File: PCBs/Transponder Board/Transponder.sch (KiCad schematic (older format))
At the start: 17 parts

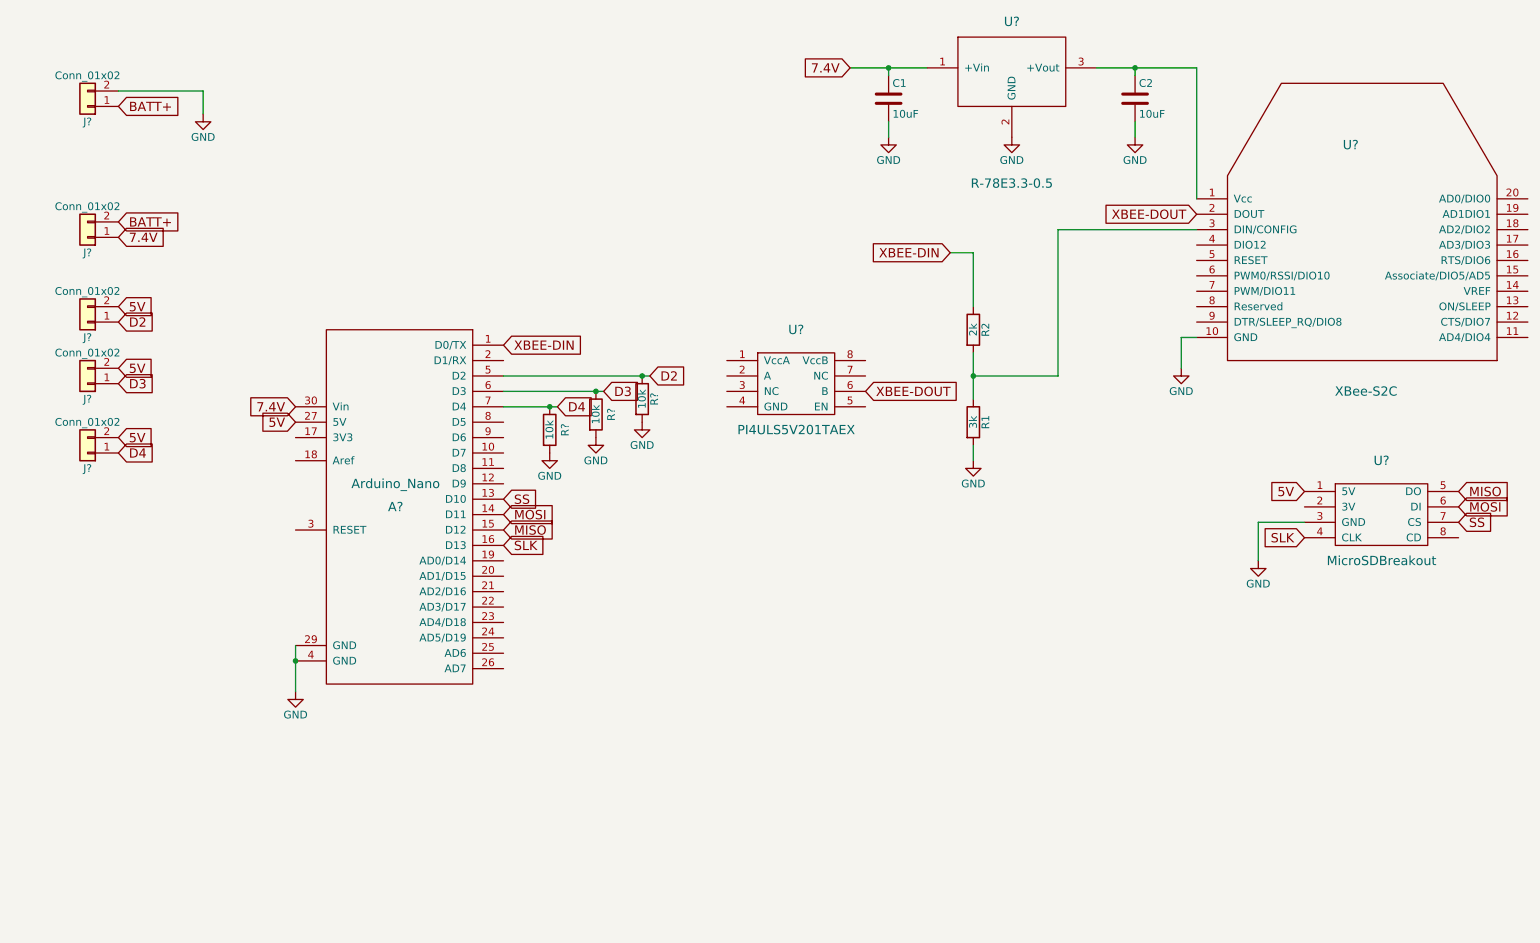
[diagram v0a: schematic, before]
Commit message: transponder board
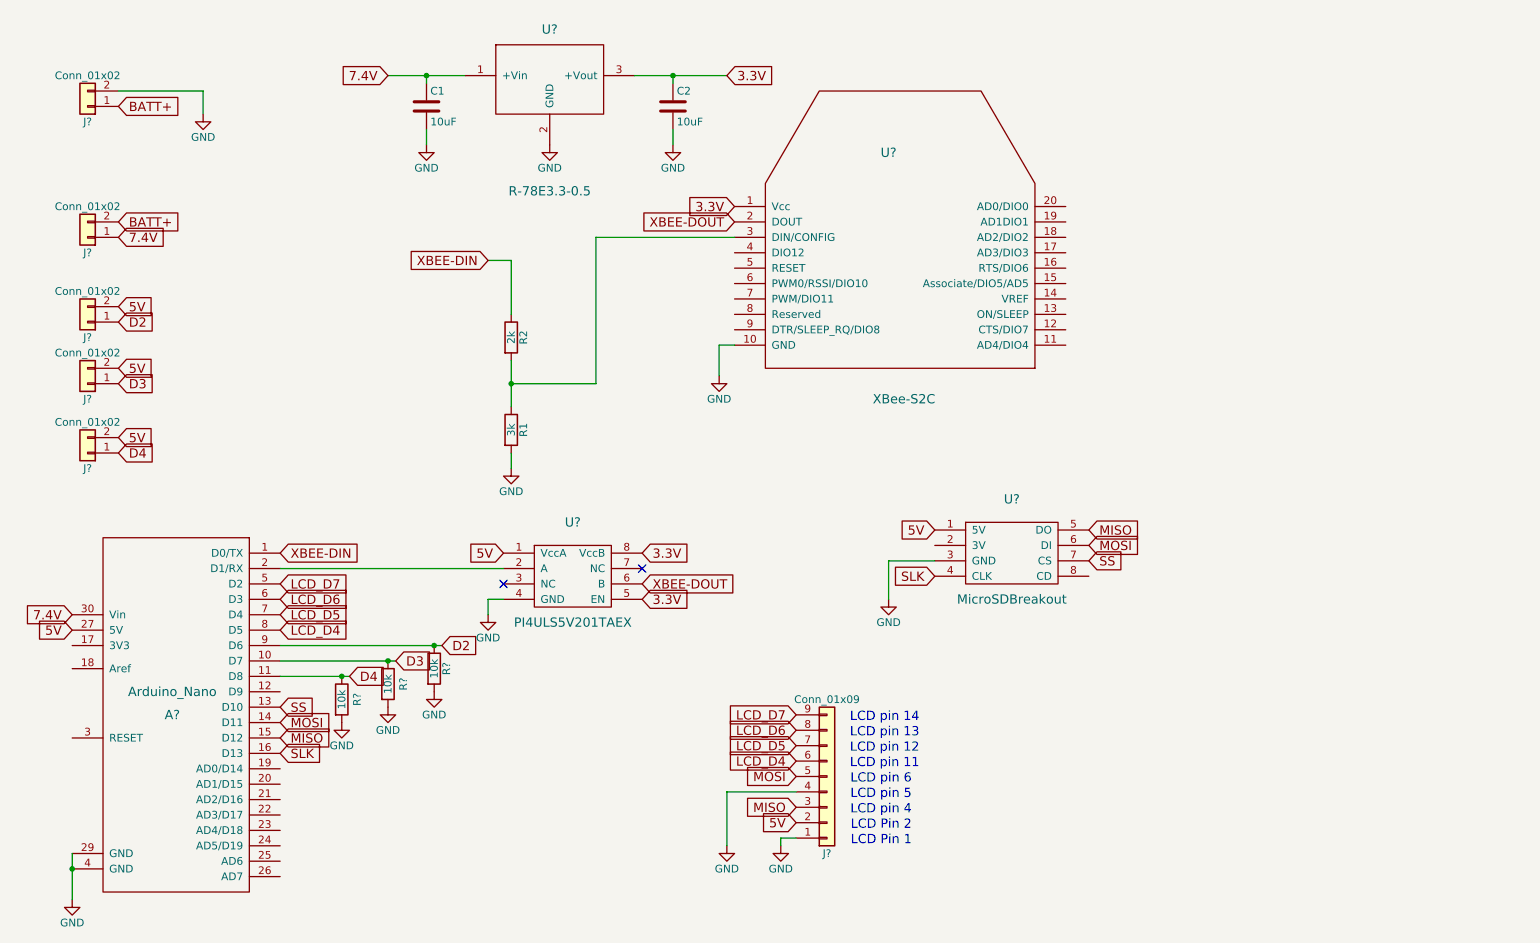
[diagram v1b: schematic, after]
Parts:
- added J?: Conn_01x09, symbol Conn_01x09
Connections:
- net 5V: now also U?.1 (VccA), J?.2 (Pin_2)
- net D2: now also A?.9 (D6); no longer A?.5 (D2)
- net D3: now also A?.10 (D7); no longer A?.6 (D3)
- net D4: now also A?.11 (D8); no longer A?.7 (D4)
- net GND: now also U?.4 (GND), J?.1 (Pin_1), J?.4 (Pin_4)
- net MISO: now also J?.3 (Pin_3)
- net MOSI: now also J?.5 (Pin_5)
- net at A?.2 (D1/RX): now also U?.2 (A)
- net LCD_D4: now reaches A?.8 (D5)
- net LCD_D4: now also J?.6 (Pin_6)
- net 3.3V: now reaches C2.1, U?.1 (Vcc), U?.3 (+Vout)
- net 3.3V: now also U?.5 (EN), U?.8 (VccB)
- new net LCD_D5: A?.7 (D4), J?.7 (Pin_7)
- new net LCD_D6: A?.6 (D3), J?.8 (Pin_8)
- new net LCD_D7: A?.5 (D2), J?.9 (Pin_9)
- no-connect marks 0 -> 2
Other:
- note added: "LCD Pin 1"
- note added: "LCD Pin 2"
- note added: "LCD pin 11"
- note added: "LCD pin 12"
- note added: "LCD pin 13"
- note added: "LCD pin 14"
- note added: "LCD pin 4"
- note added: "LCD pin 5"
- note added: "LCD pin 6"
- moved on the sheet: A?, C1, C2, R1, R2, R?, U?
